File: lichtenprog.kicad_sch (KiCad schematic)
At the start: 63 parts, among them J1 USB_C_Receptacle_USB2.0, J2 IO_OUT, SW1 VDD_RST, SW2 LIPO_RST, U1 SPX3819M5-L, U2 MCP6L04x-xSL, U3 USBLC6-2SC6, U4 CP2102N-A01-GQFN28, U5 SN74LVC1T45DBV, U6 SN74LVC1T45DBV, U7 SPX3819M5-L

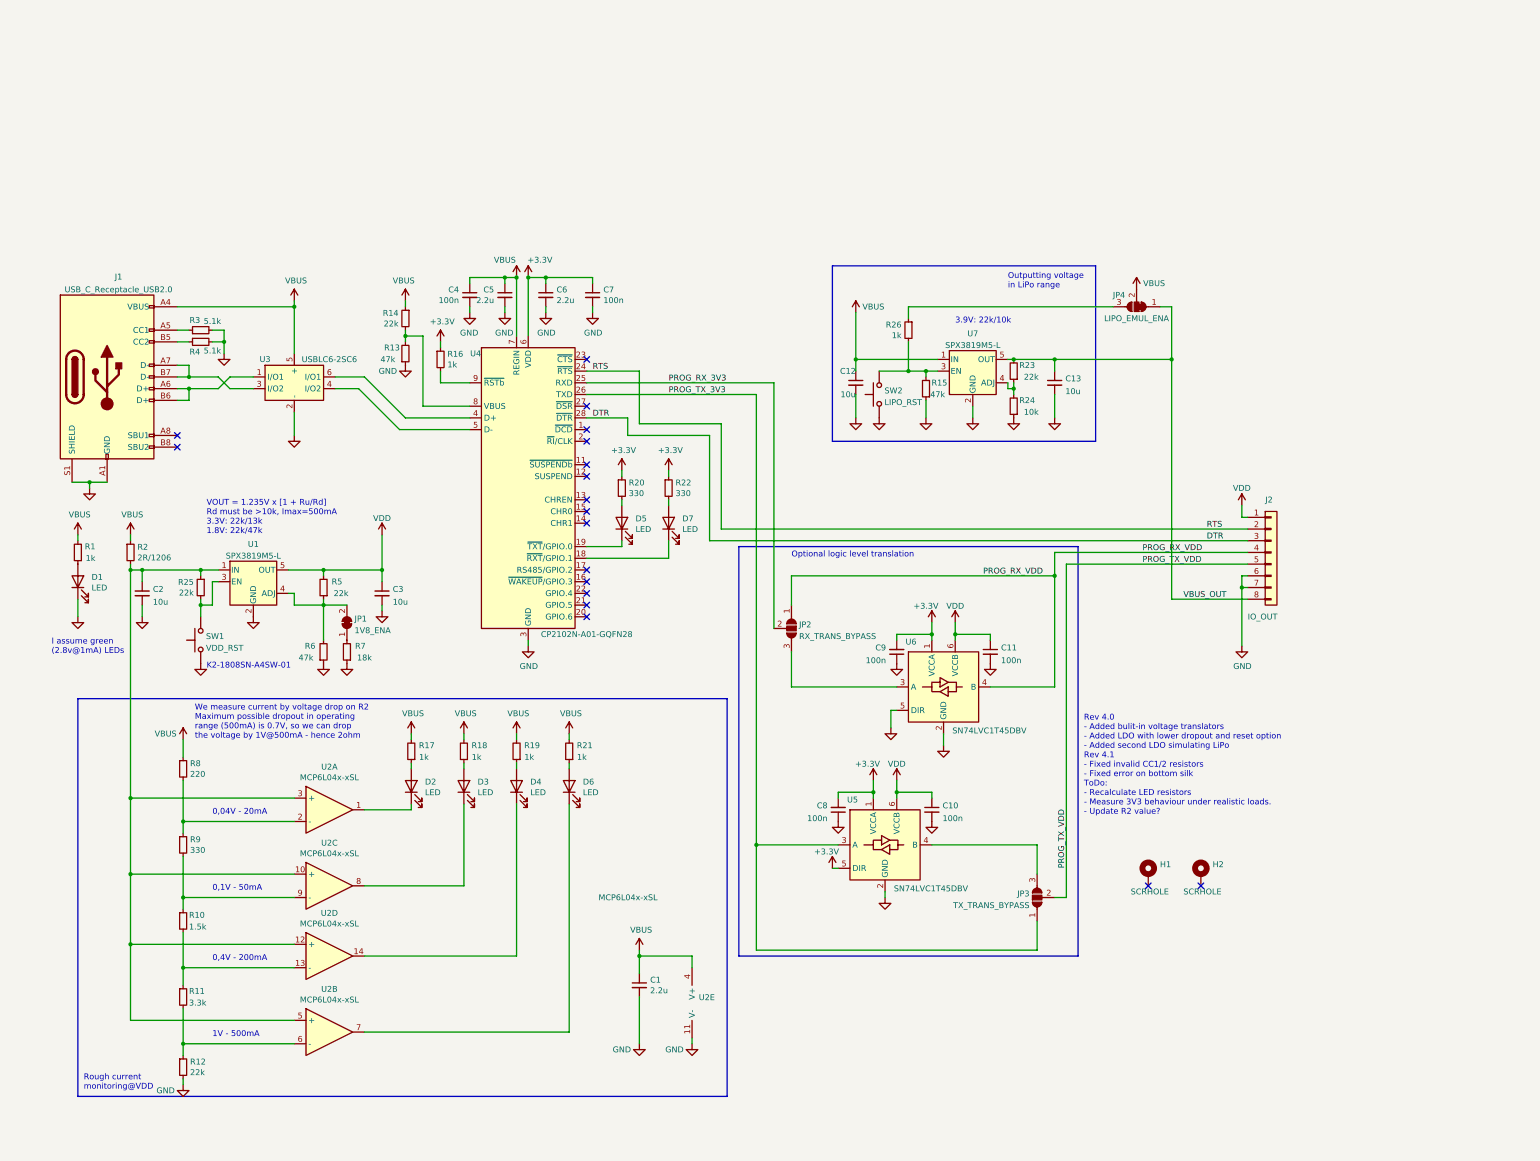
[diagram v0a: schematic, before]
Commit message: route complt
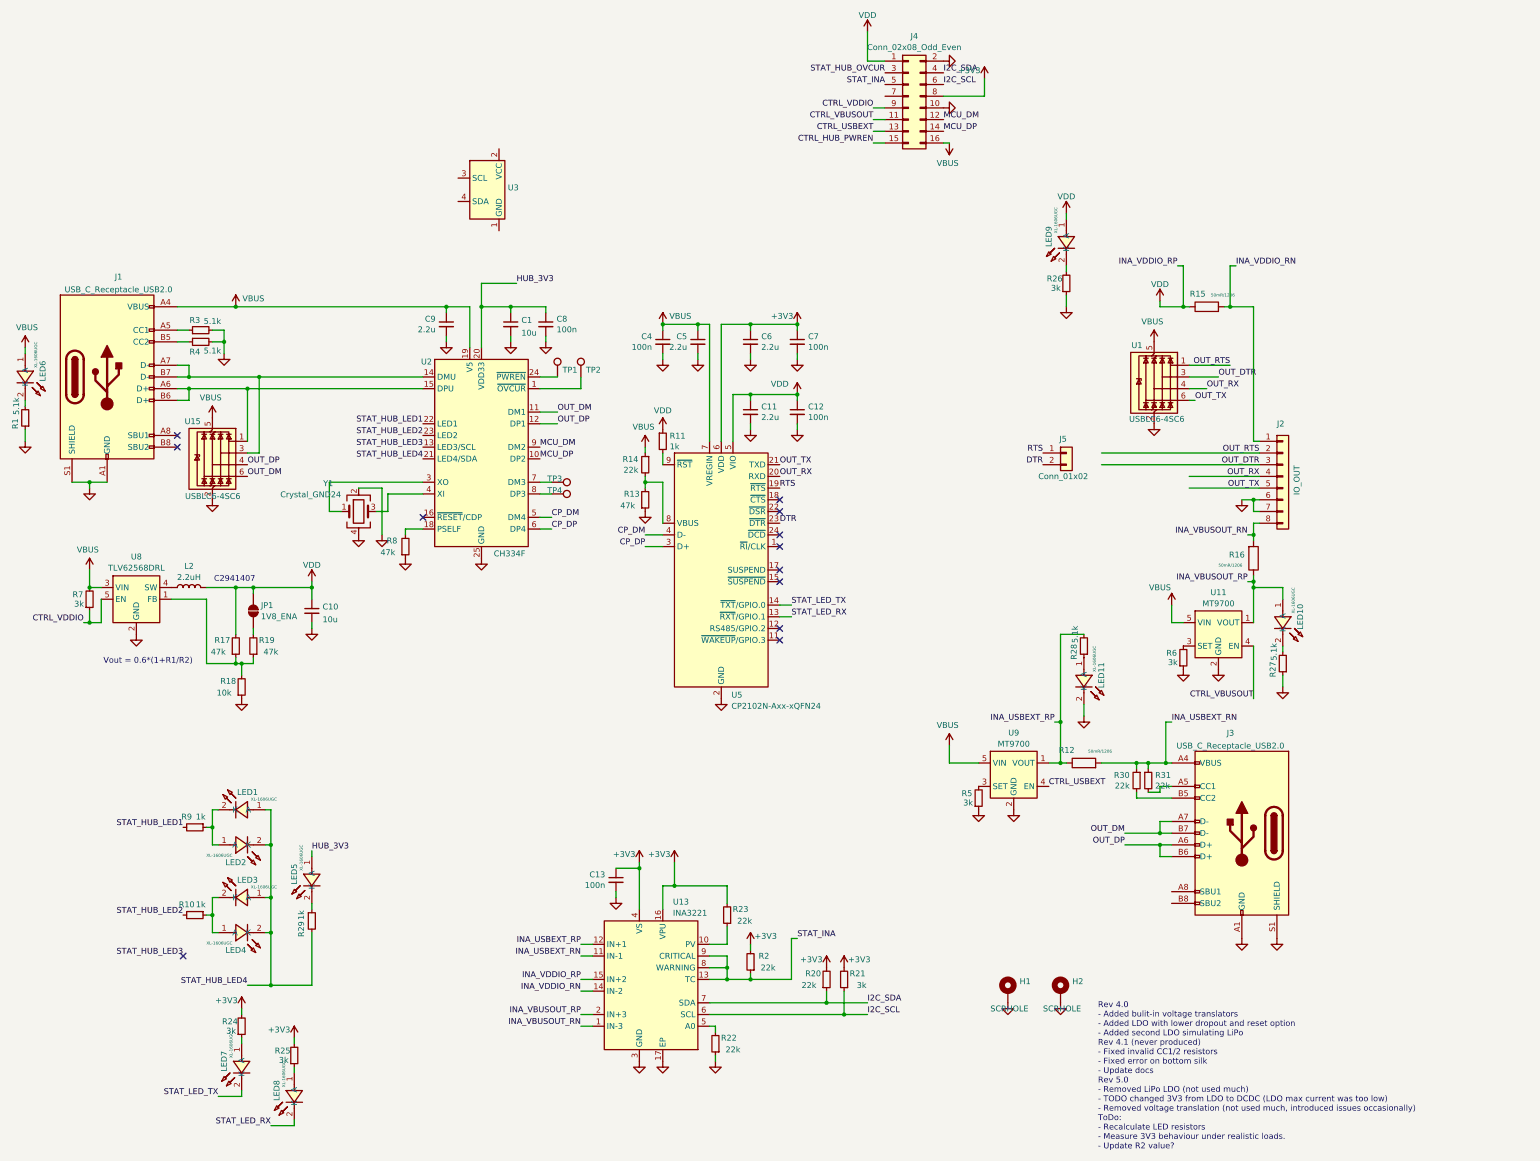
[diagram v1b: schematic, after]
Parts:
- removed C2, C3: 10u, Capacitor_SMD:C_0603_1608Metric, symbol Device:C_Small
- removed D1, D2, D3, D4, D5, D6, D7: LED, LED_SMD:LED_0603_1608Metric, symbol Device:LED
- removed JP1: 1V8_ENA, Jumper:SolderJumper-2_P1.3mm_Bridged2Bar_Pad1.0x1.5mm, symbol Jumper:SolderJumper_2_Bridged
- removed JP2: RX_TRANS_BYPASS, Jumper:SolderJumper-3_P2.0mm_Open_TrianglePad1.0x1.5mm, symbol Jumper:SolderJumper_3_Open
- removed JP3: TX_TRANS_BYPASS, Jumper:SolderJumper-3_P2.0mm_Open_TrianglePad1.0x1.5mm, symbol Jumper:SolderJumper_3_Open
- removed JP4: LIPO_EMUL_ENA, Jumper:SolderJumper-3_P2.0mm_Open_TrianglePad1.0x1.5mm, symbol Jumper:SolderJumper_3_Bridged12
- removed R12: 22k, Resistor_SMD:R_0402_1005Metric, symbol Device:R_Small
- removed R15: 47k, Resistor_SMD:R_0402_1005Metric, symbol Device:R_Small
- removed R16: 1k, Resistor_SMD:R_0402_1005Metric, symbol Device:R_Small
- removed SW1: VDD_RST, Button_Switch_SMD:SW_Push_1P1T_NO_Vertical_Wuerth_434133025816, symbol Switch:SW_Push
- removed SW2: LIPO_RST, Button_Switch_SMD:SW_Push_1P1T_NO_Vertical_Wuerth_434133025816, symbol Switch:SW_Push
- removed U1, U7: SPX3819M5-L, Package_TO_SOT_SMD:SOT-23-5, symbol Regulator_Linear:SPX3819M5-L
- removed U2: MCP6L04x-xSL, Package_SO:SOIC-14_3.9x8.7mm_P1.27mm, symbol Amplifier_Operational:MCP6L04x-xSL
- removed U3: USBLC6-2SC6, Package_TO_SOT_SMD:SOT-23-6, symbol Critbit_lib:USBLC6-2SC6
- removed U4: CP2102N-A01-GQFN28, Package_DFN_QFN:QFN-28-1EP_5x5mm_P0.5mm_EP3.35x3.35mm, symbol Interface_USB:CP2102N-A01-GQFN28
- removed U5, U6: SN74LVC1T45DBV, Package_TO_SOT_SMD:SOT-23-6, symbol Logic_LevelTranslator:SN74LVC1T45DBV
- added J3: USB_C_Receptacle_USB2.0, Connector_USB:USB_C_Receptacle_HRO_TYPE-C-31-M-12, symbol Connector:USB_C_Receptacle_USB2.0
- added J4: Conn_02x08_Odd_Even, Connector_PinSocket_1.27mm:PinSocket_2x08_P1.27mm_Vertical_SMD, symbol Connector_Generic:Conn_02x08_Odd_Even
- added J5: Conn_01x02, Connector_PinHeader_2.54mm:PinHeader_1x02_P2.54mm_Vertical, symbol Connector_Generic:Conn_01x02
- added JP1: 1V8_ENA, Jumper:SolderJumper-2_P1.3mm_Open_RoundedPad1.0x1.5mm, symbol Jumper:SolderJumper_2_Open
- added L2: 2.2uH, Inductor_SMD:L_Sunlord_MWSA0412S, symbol Device:L
- added LED1, LED10, LED11, LED2, LED3, LED4, LED5, LED6, LED7, LED8, LED9: XL-1606UGC, easyeda2kicad:LED-SMD_L1.7-W1.1-R-RD_GREEN, symbol easyeda2kicad:XL-1606UGC
- added R12, R15, R16: 50mR/1206, Resistor_SMD:R_1206_3216Metric_Pad1.30x1.75mm_HandSolder, symbol Device:R
- added R27, R28: 5.1k, Resistor_SMD:R_0402_1005Metric, symbol Device:R_Small
- added R29: 1k, Resistor_SMD:R_0402_1005Metric, symbol Device:R_Small
- added R30, R31: 22k, Resistor_SMD:R_0402_1005Metric, symbol Device:R_Small
- added TP1, TP2, TP3, TP4: TestPoint, TestPoint:TestPoint_Pad_D1.0mm, symbol Connector:TestPoint
- added U1, U15: USBLC6-4SC6, Package_TO_SOT_SMD:SOT-23-6, symbol Power_Protection:USBLC6-4SC6
- added U11, U9: MT9700, easyeda2kicad:SOT-23-5_L3.0-W1.7-P0.95-LS2.8-BR, symbol easyeda2kicad:MT9700
- added U13: INA3221, Package_DFN_QFN:Texas_RGV0016A_VQFN-16-1EP_4x4mm_P0.65mm_EP2.1x2.1mm, symbol Power_Management:INA3221
- added U2: CH334F, easyeda2kicad:QFN-24_L4.0-W4.0-P0.50-BL-EP2.8, symbol easyeda2kicad:CH334F_C5187527
- added U3: ~, Critbit_lib:OLED_4Pin_128x64_new, symbol Critbit_lib:OLED_4Pin
- added U5: CP2102N-Axx-xQFN24, Package_DFN_QFN:QFN-24-1EP_4x4mm_P0.5mm_EP2.6x2.6mm, symbol Interface_USB:CP2102N-Axx-xQFN24
- added U8: TLV62568DRL, Package_TO_SOT_SMD:SOT-563, symbol Regulator_Switching:TLV62568DRL
- added Y1: Crystal_GND24, Crystal:Crystal_SMD_3225-4Pin_3.2x2.5mm, symbol Device:Crystal_GND24
- C1: value 2.2u -> 10u; footprint Capacitor_SMD:C_0402_1005Metric -> Capacitor_SMD:C_0603_1608Metric; LCSC C12530 -> C19702
- C10: value 100n -> 10u; footprint Capacitor_SMD:C_0402_1005Metric -> Capacitor_SMD:C_0603_1608Metric; LCSC C1525 -> C19702
- C11, C9: value 100n -> 2.2u; footprint Capacitor_SMD:C_0402_1005Metric -> Capacitor_SMD:C_0603_1608Metric; LCSC C1525 -> C12530
- C12, C13: value 10u -> 100n; footprint Capacitor_SMD:C_0603_1608Metric -> Capacitor_SMD:C_0402_1005Metric; LCSC C19702 -> C1525
- C5, C6: footprint Capacitor_SMD:C_0402_1005Metric -> Capacitor_SMD:C_0603_1608Metric
- R1: value 1k -> 5.1k; LCSC C11702 -> C25117
- R10: value 1.5k -> 1k; LCSC C25867 -> C25768
- R11: value 3.3k -> 1k; LCSC C25890 -> C11702
- R17, R19: value 1k -> 47k; LCSC C11702 -> C25768
- R18: value 1k -> 10k; LCSC C11702 -> C25792
- R2: value 2R/1206 -> 22k; footprint Resistor_SMD:R_1206_3216Metric -> Resistor_SMD:R_0402_1005Metric; LCSC C17942 -> C25768
- R20, R22: value 330 -> 22k; LCSC C25104 -> C25768
- R21, R26: value 1k -> 3k; LCSC C11702 -> C25768
- R24: value 10k -> 3k; LCSC C25744 -> C25768
- R25, R5: value 22k -> 3k
- R6: value 47k -> 3k; LCSC C25792 -> C25768
- R7: value 18k -> 3k; LCSC C25762 -> C25768
- R8: value 220 -> 47k; LCSC C25091 -> C25792
- R9: value 330 -> 1k; LCSC C25104 -> C25768
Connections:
- net +3V3: now also C13.1, R2.2, R20.2, R21.2, R23.2, R24.2, R25.2, J4.8 (Pin_8), U13.16 (VPU), U13.4 (VS), U5.6 (VDD); no longer C8.2, C9.2, R20.1, R22.1
- net DTR: now also J5.2 (Pin_2), U5.23 (~{DTR}); no longer J2.3 (Pin_3)
- net GND: now also C8.2, C9.2, H1.1, H2.1, R1.1, R18.1, R22.1, R26.1, R5.1, R8.1, J3.A1 (GND), J3.A12 (GND), J3.B1 (GND), J3.B12 (GND), J3.S1 (SHIELD), J4.10 (Pin_10), J4.2 (Pin_2), LED11.2 (K), R27.1, U1.2 (GND), U11.2 (GND), U13.17 (EP), U13.3 (GND), U15.2 (GND), U2.25 (GND), U5.2 (GND), U5.25 (GND), U8.2 (GND), U9.2 (GND), Y1.2, Y1.4; no longer C8.1, C9.1, R24.1, R7.1
- net RTS: now also J5.1 (Pin_1), U5.19 (~{RTS}); no longer J2.2 (Pin_2)
- net VBUS: now also C9.1, R7.2, J4.16 (Pin_16), LED6.1 (A), U1.5 (VBUS), U11.5 (VIN), U15.5 (VBUS), U2.19 (V5), U5.7 (VREGIN), U8.3 (VIN), U9.5 (VIN); no longer C1.1, C12.1, R1.2, R17.2, R18.2, R19.2, R2.1, R21.2, R8.1
- net VDD: now also C12.1, R11.1, R17.2, J4.1 (Pin_1), JP1.2 (B), L2.2, LED9.1 (A), R15.1, U13.15 (IN+2), U5.5 (VIO); no longer J2.1 (Pin_1), R5.2
- net at R13.2, R14.2: now also U5.8 (VBUS)
- net at R22.2: now also U13.5 (A0)
- net at R25.1: now also LED8.1 (A); no longer R2.2
- net at R11.2: now also U5.9 (~{RST})
- net STAT_HUB_LED2: now reaches R10.2
- net STAT_HUB_LED2: now also U2.23 (LED2); no longer R11.1
- net at R10.1: now also LED3.2 (K), LED4.1 (A); no longer R9.2
- net at R9.1: now also LED1.2 (K), LED2.1 (A); no longer R8.2
- net at R17.1: now also R18.2, R19.1, U8.1 (FB)
- net I2C_SCL: now reaches R21.1
- net I2C_SCL: now also J4.6 (Pin_6), U13.6 (SCL)
- net at R6.2: now also U11.3 (SET); no longer R5.1
- net at J1.A6 (D+), J1.B6 (D+): now also U15.1 (I/O1), U2.15 (DPU)
- net at J1.A7 (D-), J1.B7 (D-): now also U15.3 (I/O2), U2.14 (DMU)
- net at R26.2: now also LED9.2 (K)
- net at R23.1: now also U13.10 (PV); no longer R24.2
- net PROG_RX_VDD renamed OUT_RX
- net OUT_RX: now also U1.4 (I/O3), U5.20 (RXD)
- net PROG_TX_VDD renamed OUT_TX
- net OUT_TX: now also U1.6 (I/O4), U5.21 (TXD)
- removed net VBUS_OUT: C13.1, J2.8 (Pin_8), R23.2
- new net: LED7.1 (A), R24.1
- new net: LED11.1 (A), R28.1
- new net: JP1.1 (A), R19.2
- new net: TP3.1, U2.7 (DM3)
- new net: LED5.2 (K), R29.1
- new net: TP1.1, U2.24 (~{PWREN})
- new net: R8.2, U2.18 (PSELF)
- new net: TP2.1, U2.1 (~{OVCUR})
- new net: J3.B5 (CC2), R30.2
- new net: LED6.2 (K), R1.2
- new net: R5.2, U9.3 (SET)
- new net: J3.A5 (CC1), R31.2
- new net: LED10.2 (K), R27.2
- new net: L2.1, U8.4 (SW)
- new net: TP4.1, U2.8 (DP3)
- new net: U2.3 (XO), Y1.1
- new net: U2.4 (XI), Y1.3
- new net CP_DM: U2.5 (DM4), U5.4 (D-)
- new net CP_DP: U2.6 (DP4), U5.3 (D+)
- new net CTRL_HUB_PWREN: J4.15 (Pin_15)
- new net CTRL_USBEXT: J4.13 (Pin_13), U9.4 (EN)
- new net CTRL_VBUSOUT: J4.11 (Pin_11), U11.4 (EN)
- new net CTRL_VDDIO: J4.9 (Pin_9), R7.1, U8.5 (EN)
- new net HUB_3V3: C1.1, C8.1, LED5.1 (A), U2.20 (VDD33)
- new net I2C_SDA: J4.4 (Pin_4), R20.1, U13.7 (SDA)
- new net INA_USBEXT_RN: J3.A4 (VBUS), J3.A9 (VBUS), J3.B4 (VBUS), J3.B9 (VBUS), R12.2, R30.1, R31.1, U13.11 (IN-1)
- new net INA_USBEXT_RP: R12.1, R28.2, U13.12 (IN+1), U9.1 (VOUT)
- new net INA_VBUSOUT_RN: J2.8 (Pin_8), R16.2, U13.1 (IN-3)
- new net INA_VBUSOUT_RP: LED10.1 (A), R16.1, U11.1 (VOUT), U13.2 (IN+3)
- new net INA_VDDIO_RN: J2.1 (Pin_1), R15.2, U13.14 (IN-2)
- new net MCU_DM: J4.12 (Pin_12), U2.9 (DM2)
- new net MCU_DP: J4.14 (Pin_14), U2.10 (DP2)
- new net OUT_DM: J3.A7 (D-), J3.B7 (D-), U15.6 (I/O4), U2.11 (DM1)
- new net OUT_DP: J3.A6 (D+), J3.B6 (D+), U15.4 (I/O3), U2.12 (DP1)
- new net OUT_DTR: J2.3 (Pin_3), U1.3 (I/O2)
- new net OUT_RTS: J2.2 (Pin_2), U1.1 (I/O1)
- new net STAT_HUB_LED1: R9.2, U2.22 (LED1)
- new net STAT_HUB_LED3: U2.13 (LED3/SCL)
- new net STAT_HUB_LED4: LED1.1 (A), LED2.2 (K), LED3.1 (A), LED4.2 (K), R29.2, U2.21 (LED4/SDA)
- new net STAT_HUB_OVCUR: J4.3 (Pin_3)
- new net STAT_INA: J4.5 (Pin_5), R2.1, U13.13 (TC), U13.8 (WARNING), U13.9 (CRITICAL)
- new net STAT_LED_RX: LED8.2 (K), U5.13 (~{RXT}/GPIO.1)
- new net STAT_LED_TX: LED7.2 (K), U5.14 (~{TXT}/GPIO.0)
- no-connect marks 18 -> 12
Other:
- note added: "C2941407"
- note added: "Rev 4.0 - Added bulit-in voltage translators - Added LDO with lower dropout and reset option - Added second LDO simulating LiPo Rev 4.1 (never produced) - Fixed invalid CC1/2 resistors - Fixed error on bottom silk - Update docs Rev 5.0 - Removed LiPo LDO (not used much) - TODO changed 3V3 from LDO to DCDC (LDO max current was too low) - Removed voltage translation (not used much, introduced issue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"
- note added: "Vout = 0.6*(1+R1/R2)"
- note removed: "0,04V - 20mA"
- note removed: "0,1V - 50mA"
- note removed: "0,4V - 200mA"
- note removed: "1V - 500mA"
- note removed: "3.9V: 22k/10k"
- note removed: "I assume green (2.8v@1mA) LEDs"
- note removed: "K2-1808SN-A4SW-01"
- note removed: "Optional logic level translation"
- note removed: "Outputting voltage in LiPo range"
- note removed: "Rev 4.0 - Added bulit-in voltage translators - Added LDO with lower dropout and reset option - Added second LDO simulating LiPo Rev 4.1 - Fixed invalid CC1/2 resistors - Fixed error on bottom silk ToDo: - Recalculate LED resistors - Measure 3V3 behaviour under realistic loads. - Update R2 value?"
- note removed: "Rough current monitoring@VDD"
- note removed: "VOUT = 1.235V x [1 + Ru/Rd] Rd must be >10k, Imax=500mA 3.3V: 22k/13k 1.8V: 22k/47k"
- note removed: "We measure current by voltage drop on R2 Maximum possible dropout in operating range (500mA) is 0.7V, so we can drop the voltage by 1V@500mA - hence 2ohm"
- moved on the sheet: C4, C5, C6, C7, H1, H2, J2, R13, R14
